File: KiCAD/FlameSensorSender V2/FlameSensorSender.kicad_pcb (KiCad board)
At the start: 2 copper layers, 91 x 84 mm, 50 parts, among them IC1 LM66200DRLR, J1 SWD, J2 SWD, J3 Conn_01x06_Socket, J5 Conn_01x01_Socket, J6 Conn_01x01_Socket, J7 Conn_01x06_Socket, P1 XL638020, P2 XL638020, Q1 AO3401A, Q2 AO3400A, Q3 AO3401A, Q4 AO3400A, Q5 AO3400A, Q6 AO3401A, SW1 SW_Push, SW2 SW_Push, U1 STM32F103C8Tx, U2 Ra-01SCH-P, U3 TVS0500DRV

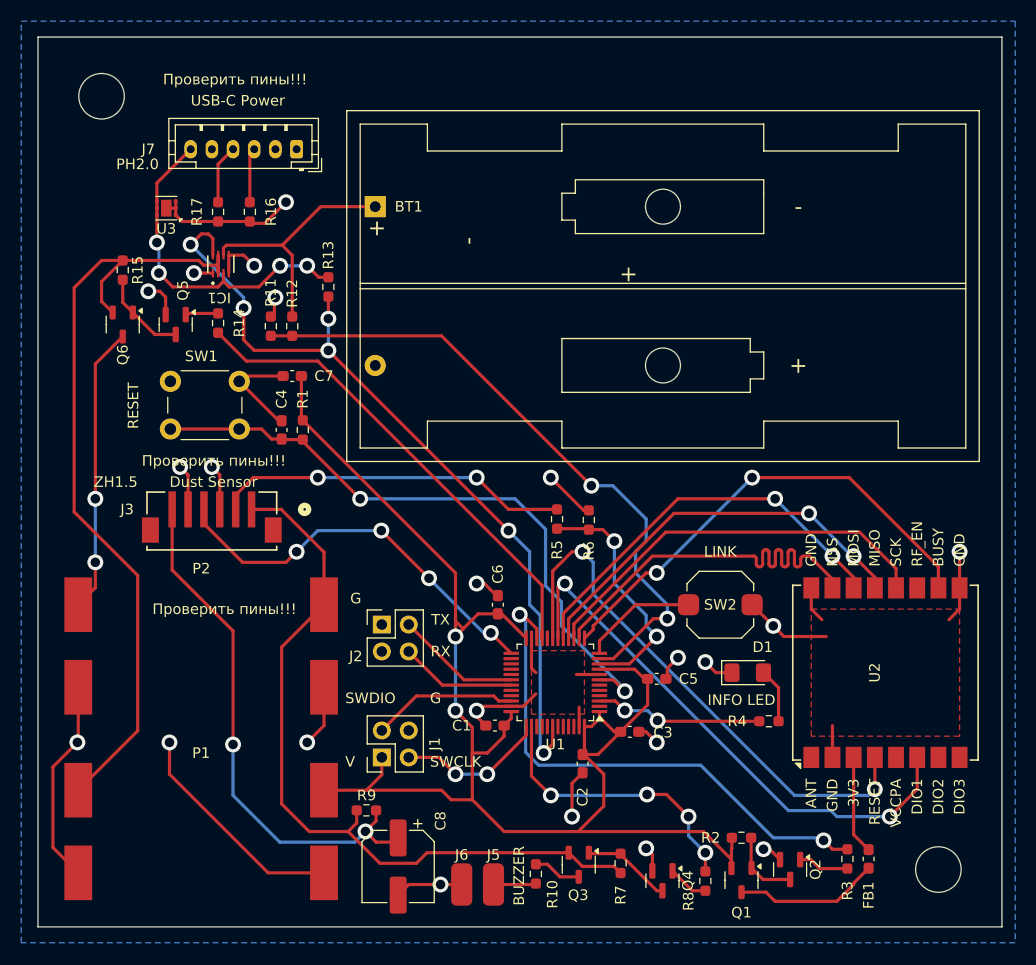
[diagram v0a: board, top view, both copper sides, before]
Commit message: dev
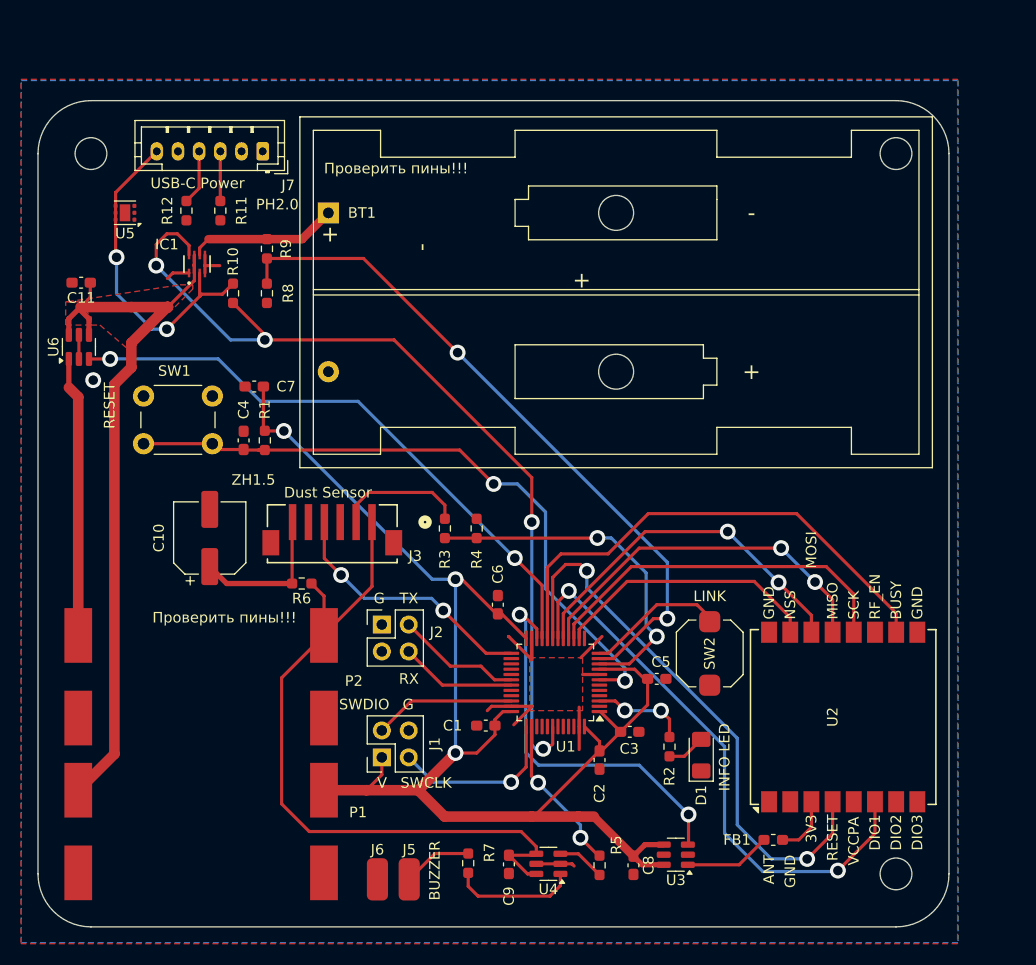
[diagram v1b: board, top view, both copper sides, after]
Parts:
- removed Q1, Q3, Q6: AO3401A, Package_TO_SOT_SMD:SOT-23-3
- removed Q2, Q4, Q5: AO3400A, Package_TO_SOT_SMD:SOT-23
- removed R14: 10,0603, Resistor_SMD:R_0603_1608Metric_Pad0.98x0.95mm_HandSolder
- removed R15: 10k,0603, Resistor_SMD:R_0603_1608Metric_Pad0.98x0.95mm_HandSolder
- removed the R2 at (128.0, 113.0)
- removed the R3 at (138.0, 115.0)
- removed the R7 at (116.6, 115.4)
- removed the REF** at (146.6, 116.0)
- removed the REF** at (67.6, 43.0)
- added C11: 1uF,0603, Capacitor_SMD:C_0603_1608Metric_Pad1.08x0.95mm_HandSolder, F.Cu at (65.7, 60.6)
- added C8: 1uF,0603, Capacitor_SMD:C_0603_1608Metric_Pad1.08x0.95mm_HandSolder, F.Cu at (117.8, 115.6)
- added C9: 1uF,0603, Capacitor_SMD:C_0603_1608Metric_Pad1.08x0.95mm_HandSolder, F.Cu at (106.0, 115.5)
- added REF**: MountingHole_3mm, MountingHole:MountingHole_3mm, F.Cu at (66.6, 48.4)
- added REF**: MountingHole_3mm, MountingHole:MountingHole_3mm, F.Cu at (142.6, 48.4)
- added REF**: MountingHole_3mm, MountingHole:MountingHole_3mm, F.Cu at (142.6, 116.4)
- added U3: TPS22929D, Package_TO_SOT_SMD:SOT-23-6, F.Cu at (121.8, 114.6)
- added U4: TPS22929D, Package_TO_SOT_SMD:SOT-23-6, F.Cu at (109.8, 115.5)
- added U6: TPS22929D, Package_TO_SOT_SMD:SOT-23-6, F.Cu at (65.5, 66.7)
- R5: renamed from R8; value 10,0603 -> 10k,0603
- moved C10 35.8 mm to (77.8, 84.7), turned to 90 degrees
- moved R6 22.3 mm to (86.5, 89.0), turned to 180 degrees
- moved J3 11.4 mm to (89.4, 84.3)
- moved R3 10.6 mm to (100.0, 83.8)
- moved R4 10.6 mm to (103.0, 83.8)
- moved R5 10.1 mm to (114.6, 115.6), turned to -90 degrees
- moved R2 9.69 mm to (121.2, 104.4), turned to -90 degrees
- moved FB1 9.18 mm to (131.0, 113.2), turned to 0 degrees
- moved R10 9.02 mm to (80.0, 61.6)
- moved D1 8.94 mm to (124.2, 105.2), turned to 90 degrees
- moved J5 7.97 mm to (96.6, 116.9)
- moved J6 7.97 mm to (93.6, 116.9)
- moved R9 7.69 mm to (83.2, 57.4)
- moved R7 6.47 mm to (102.2, 115.4), turned to 90 degrees
- moved U2 5.78 mm to (137.6, 101.6)
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- renumbered C8 to C10, R13 to R10, R16 to R11, R17 to R12, R4 to R2, R5 to R3, R6 to R4, R9 to R6, R10 to R7, R11 to R8, R12 to R9, U3 to U5
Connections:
- R5 pad 1: Net-(Q4-G) -> /BUZZER
- R5 pad 2: /BUZZER -> Net-(U4-ON)
- U1 pad 13: /LORA_BUSY -> unconnected-(U1-PA3-Pad13)
- U1 pad 20: unconnected-(U1-PB2-Pad20) -> /LORA_BUSY
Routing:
- net GNDD: track 153.8 -> 31.7 mm, vias 22 -> 1
- net /V-LED: track 49.6 -> 14.2 mm, vias 2 -> 0
- net /Vo: track 32.3 -> 12.3 mm, vias 2 -> 0
- net /LORA_NSS: track 39.1 -> 25.5 mm
- net /MOSFET_GATE_LORA: track 50.5 -> 36.9 mm
- net /BUZZER: track 27.0 -> 14.8 mm, vias 4 -> 2
- net /SENSOR_LED: track 36.6 -> 24.8 mm, vias 4 -> 2
- net MOSFET_GATE_SENSOR: track 45.5 -> 56.6 mm, vias 0 -> 2
- net /SENSOR DATA Vo: track 22.9 -> 33.3 mm
- net Net-(BT1-+): track 23.7 -> 14.2 mm
- net Net-(Q5-D): track 8.39 -> 0.00 mm
- net Net-(Q3-G): track 8.28 -> 0.00 mm
- net +3V3: track 142.6 -> 135.0 mm, vias 2 -> 3
- net Net-(U4-VOUT): track 4.54 -> 11.9 mm
- net Net-(Q1-G): track 6.91 -> 0.00 mm
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- added copper zone on F.Cu, net VRAW
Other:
- board size 91 x 84 mm -> 86 x 78 mm
